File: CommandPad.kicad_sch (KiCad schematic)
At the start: 18 parts, among them J1 OLED_128x32, SW1 RotaryEncoder_Switch, U1 XIAO-RP2040-DIP

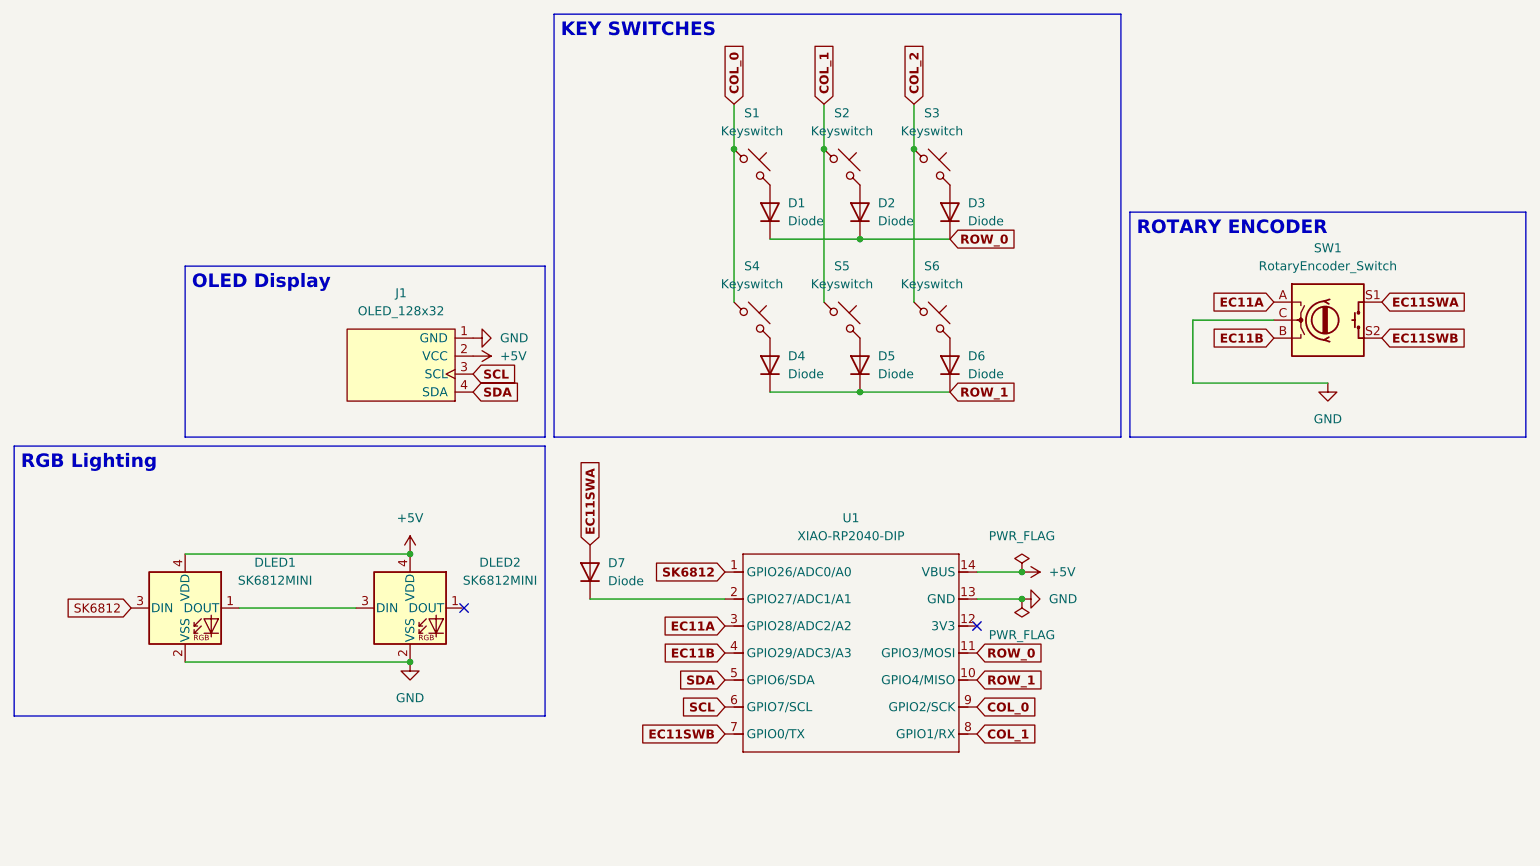
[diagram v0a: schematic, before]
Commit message: Finalized PCB design
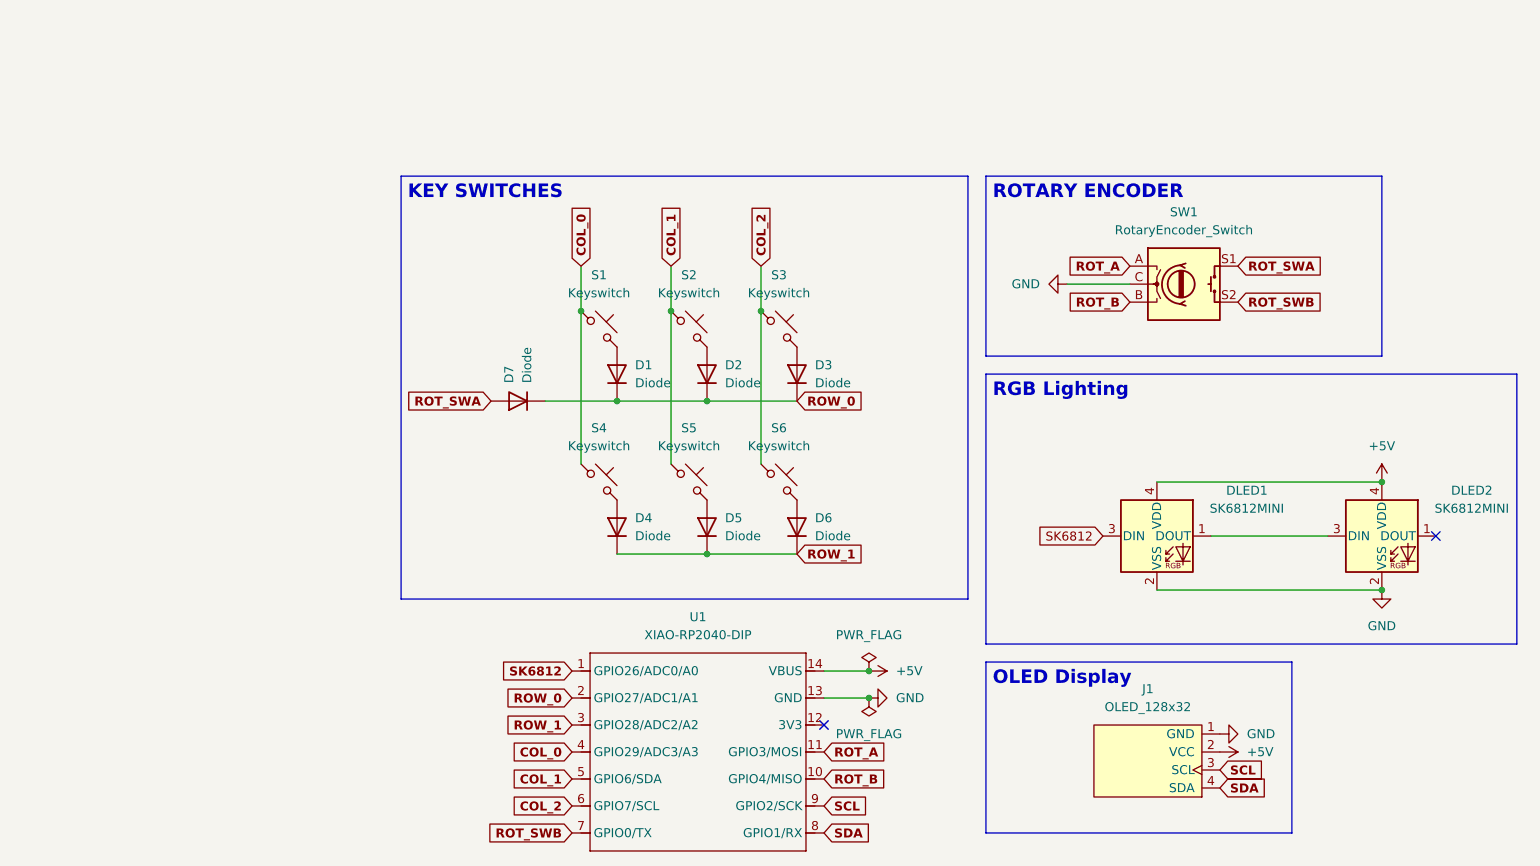
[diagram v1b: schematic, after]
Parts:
- D1, D2, D3, D4, D5, D6, D7: footprint Diode_THT:D_DO-35_SOD27_P7.62mm_Horizontal -> ScottoKeebs_Components:Diode_DO-35
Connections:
- net COL_0: now also U1.4 (GPIO29/ADC3/A3); no longer U1.9 (GPIO2/SCK)
- net COL_1: now also U1.5 (GPIO6/SDA); no longer U1.8 (GPIO1/RX)
- net COL_2: now also U1.6 (GPIO7/SCL)
- net ROW_0: now also D7.1 (K), U1.2 (GPIO27/ADC1/A1); no longer U1.11 (GPIO3/MOSI)
- net ROW_1: now also U1.3 (GPIO28/ADC2/A2); no longer U1.10 (GPIO4/MISO)
- net SCL: now also U1.9 (GPIO2/SCK); no longer U1.6 (GPIO7/SCL)
- net SDA: now also U1.8 (GPIO1/RX); no longer U1.5 (GPIO6/SDA)
- net EC11A renamed ROT_A
- net ROT_A: now also U1.11 (GPIO3/MOSI); no longer U1.3 (GPIO28/ADC2/A2)
- net EC11B renamed ROT_B
- net ROT_B: now also U1.10 (GPIO4/MISO); no longer U1.4 (GPIO29/ADC3/A3)
- net EC11SWA renamed ROT_SWA
- net EC11SWB renamed ROT_SWB
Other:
- moved on the sheet: D1, D2, D3, D4, D5, D6, D7, DLED1, DLED2, J1, S1, S2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
